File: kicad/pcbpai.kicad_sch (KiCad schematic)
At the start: 16 parts, among them J1 Fuse, J2 Conn_01x04_Pin, J3 Input 24 V, J4 Boton Encendido, J5 Parada de Emergencia, J6 Conn_01x06_Pin, J7 Raspberry GPIO, J8 Conn_01x09_Pin, J9 Conn_01x02_Socket, SW1 SW_Push_DPDT, U6 ATtiny85-20P

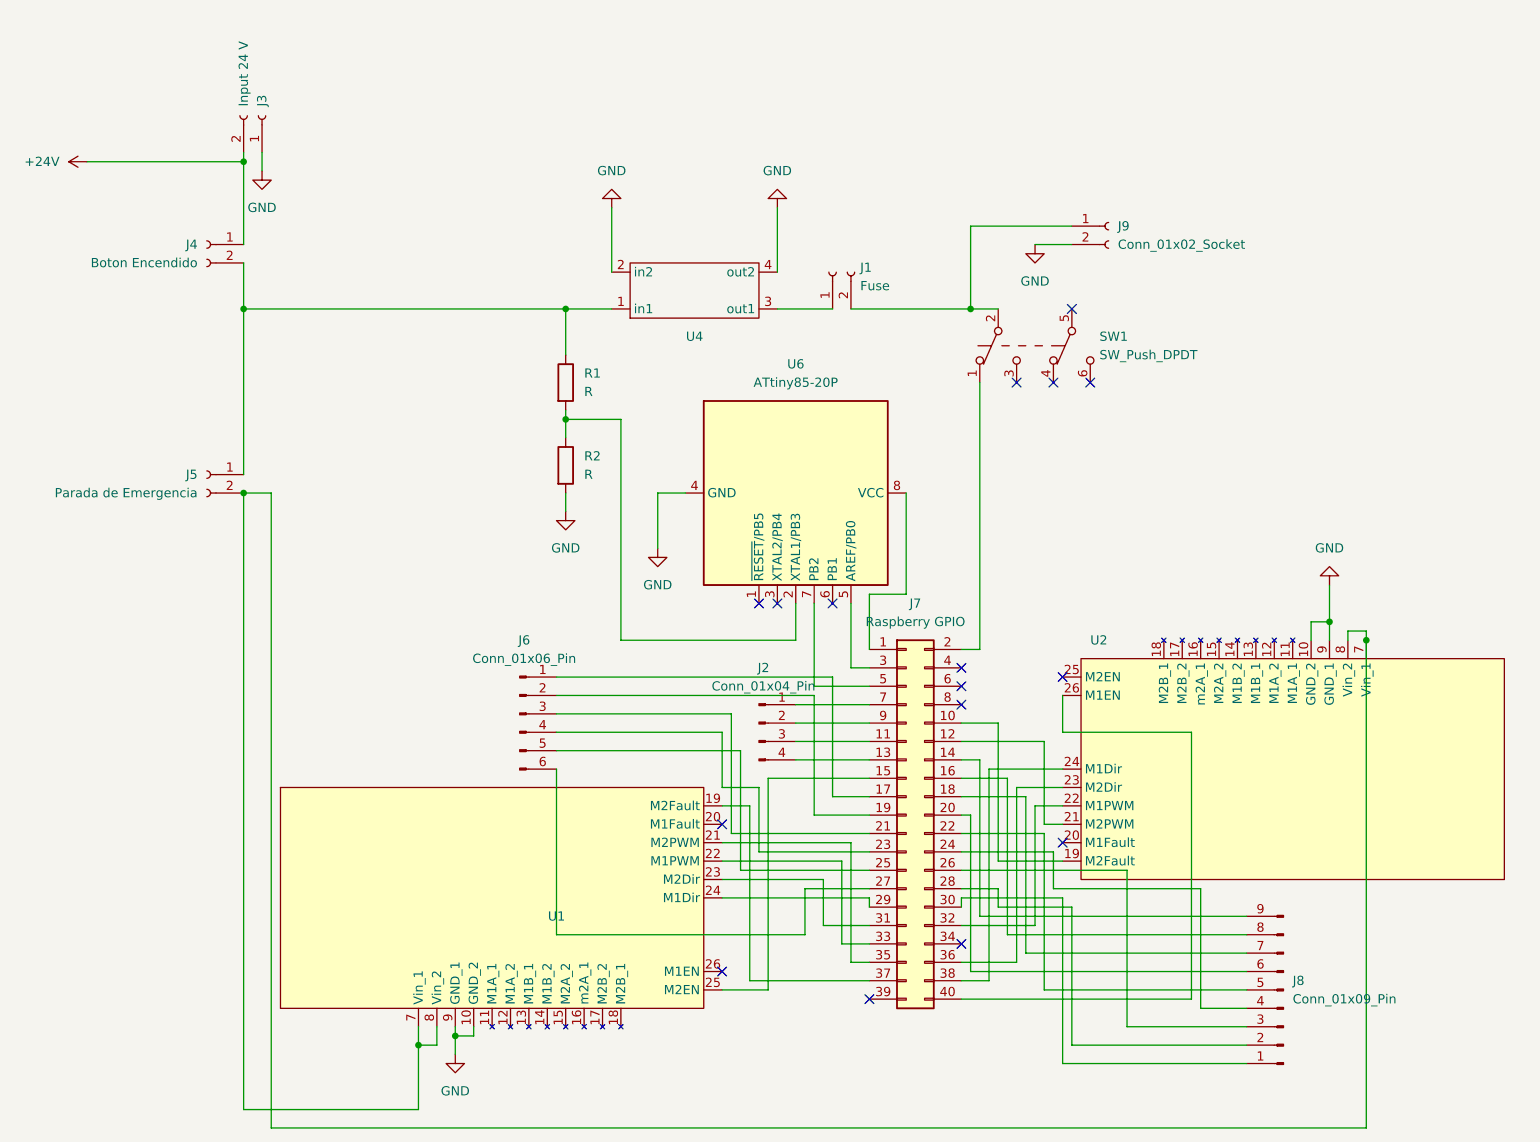
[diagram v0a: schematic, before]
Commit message: finish pcb
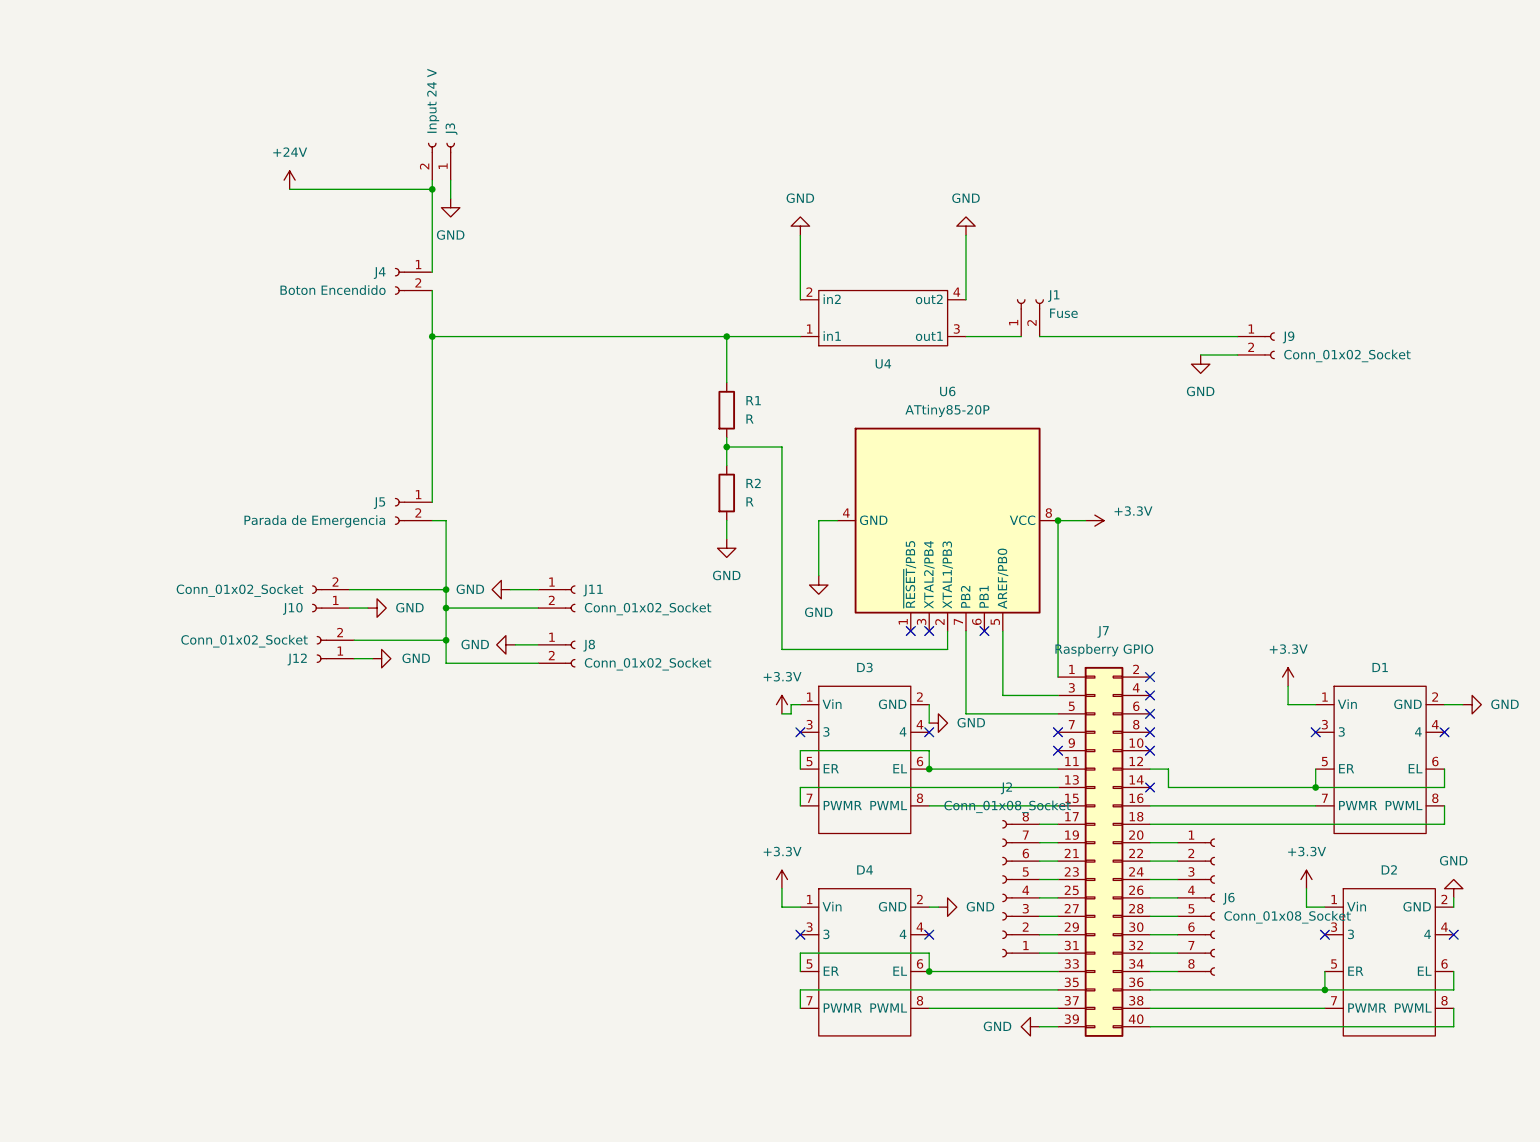
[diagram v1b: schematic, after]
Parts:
- removed J2: Conn_01x04_Pin, Connector_PinSocket_2.54mm:PinSocket_1x04_P2.54mm_Vertical, symbol Connector:Conn_01x04_Pin
- removed J6: Conn_01x06_Pin, Connector_PinSocket_2.54mm:PinSocket_1x06_P2.54mm_Vertical, symbol Connector:Conn_01x06_Pin
- removed J8: Conn_01x09_Pin, Connector_PinSocket_2.54mm:PinSocket_1x09_P2.54mm_Vertical, symbol Connector:Conn_01x09_Pin
- removed SW1: SW_Push_DPDT, PAI:switch, symbol Switch:SW_Push_DPDT
- removed U1, U2: ~, PAI:Pololu MAX 14870 Dual Shield Arduino, symbol Lib_PAI:Dual_MAX14870
- added D1, D2, D3, D4: ~, Connector_PinHeader_2.54mm:PinHeader_2x04_P2.54mm_Vertical, symbol Lib_PAI:Conector_2x4
- added J10, J11, J12, J8: Conn_01x02_Socket, Connector_Phoenix_MSTB:PhoenixContact_MSTBA_2,5_2-G_1x02_P5.00mm_Horizontal, symbol Connector:Conn_01x02_Socket
- added J2, J6: Conn_01x08_Socket, Connector_PinSocket_2.54mm:PinSocket_1x08_P2.54mm_Vertical, symbol Connector:Conn_01x08_Socket
- U4: footprint PAI:regulador -> PAI:regulator
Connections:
- net GND: now also J7.39 (Pin_39), D1.2 (GND), D2.2 (GND), D3.2 (GND), D4.2 (GND), J10.1 (Pin_1), J11.1 (Pin_1), J12.1 (Pin_1), J8.1 (Pin_1)
- net at J5.2 (Pin_2): now also J10.2 (Pin_2), J11.2 (Pin_2), J12.2 (Pin_2), J8.2 (Pin_2)
- net at J7.37 (Pin_37): now also D4.8 (PWML)
- net at J7.35 (Pin_35): now also D4.7 (PWMR)
- net at J7.33 (Pin_33): now also D4.5 (ER), D4.6 (EL)
- net at J7.31 (Pin_31): now also J2.1 (Pin_1)
- net at J7.29 (Pin_29): now also J2.2 (Pin_2)
- net at J7.15 (Pin_15): now also D3.8 (PWML)
- net at J7.12 (Pin_12): now also D1.5 (ER), D1.6 (EL)
- net at J7.32 (Pin_32): now also J6.7 (Pin_7)
- net at J7.36 (Pin_36): now also D2.5 (ER), D2.6 (EL)
- net at J7.38 (Pin_38): now also D2.7 (PWMR)
- net at J7.40 (Pin_40): now also D2.8 (PWML)
- net +3.3V: now reaches J7.1 (Pin_1), U6.8 (VCC)
- net +3.3V: now also D1.1 (Vin), D2.1 (Vin), D3.1 (Vin), D4.1 (Vin)
- net at J7.11 (Pin_11): now also D3.5 (ER), D3.6 (EL)
- net at J7.13 (Pin_13): now also D3.7 (PWMR)
- net at J7.16 (Pin_16): now also D1.7 (PWMR)
- net at J7.17 (Pin_17): now also J2.8 (Pin_8)
- net at J7.18 (Pin_18): now also D1.8 (PWML)
- net at J7.19 (Pin_19): now also J2.7 (Pin_7)
- net at J7.20 (Pin_20): now also J6.1 (Pin_1)
- net at J7.21 (Pin_21): now also J2.6 (Pin_6)
- net at J7.22 (Pin_22): now also J6.2 (Pin_2)
- net at J7.23 (Pin_23): now also J2.5 (Pin_5)
- net at J7.24 (Pin_24): now also J6.3 (Pin_3)
- net at J7.25 (Pin_25): now also J2.4 (Pin_4)
- net at J7.26 (Pin_26): now also J6.4 (Pin_4)
- net at J7.27 (Pin_27): now also J2.3 (Pin_3)
- net at J7.28 (Pin_28): now also J6.5 (Pin_5)
- net at J7.30 (Pin_30): now also J6.6 (Pin_6)
- net at J7.34 (Pin_34): now also J6.8 (Pin_8)
- no-connect marks 16 -> 19
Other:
- moved on the sheet: J1, J3, J4, J5, J7, J9, R1, R2, U4, U6

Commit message: add gerber files and change footprints
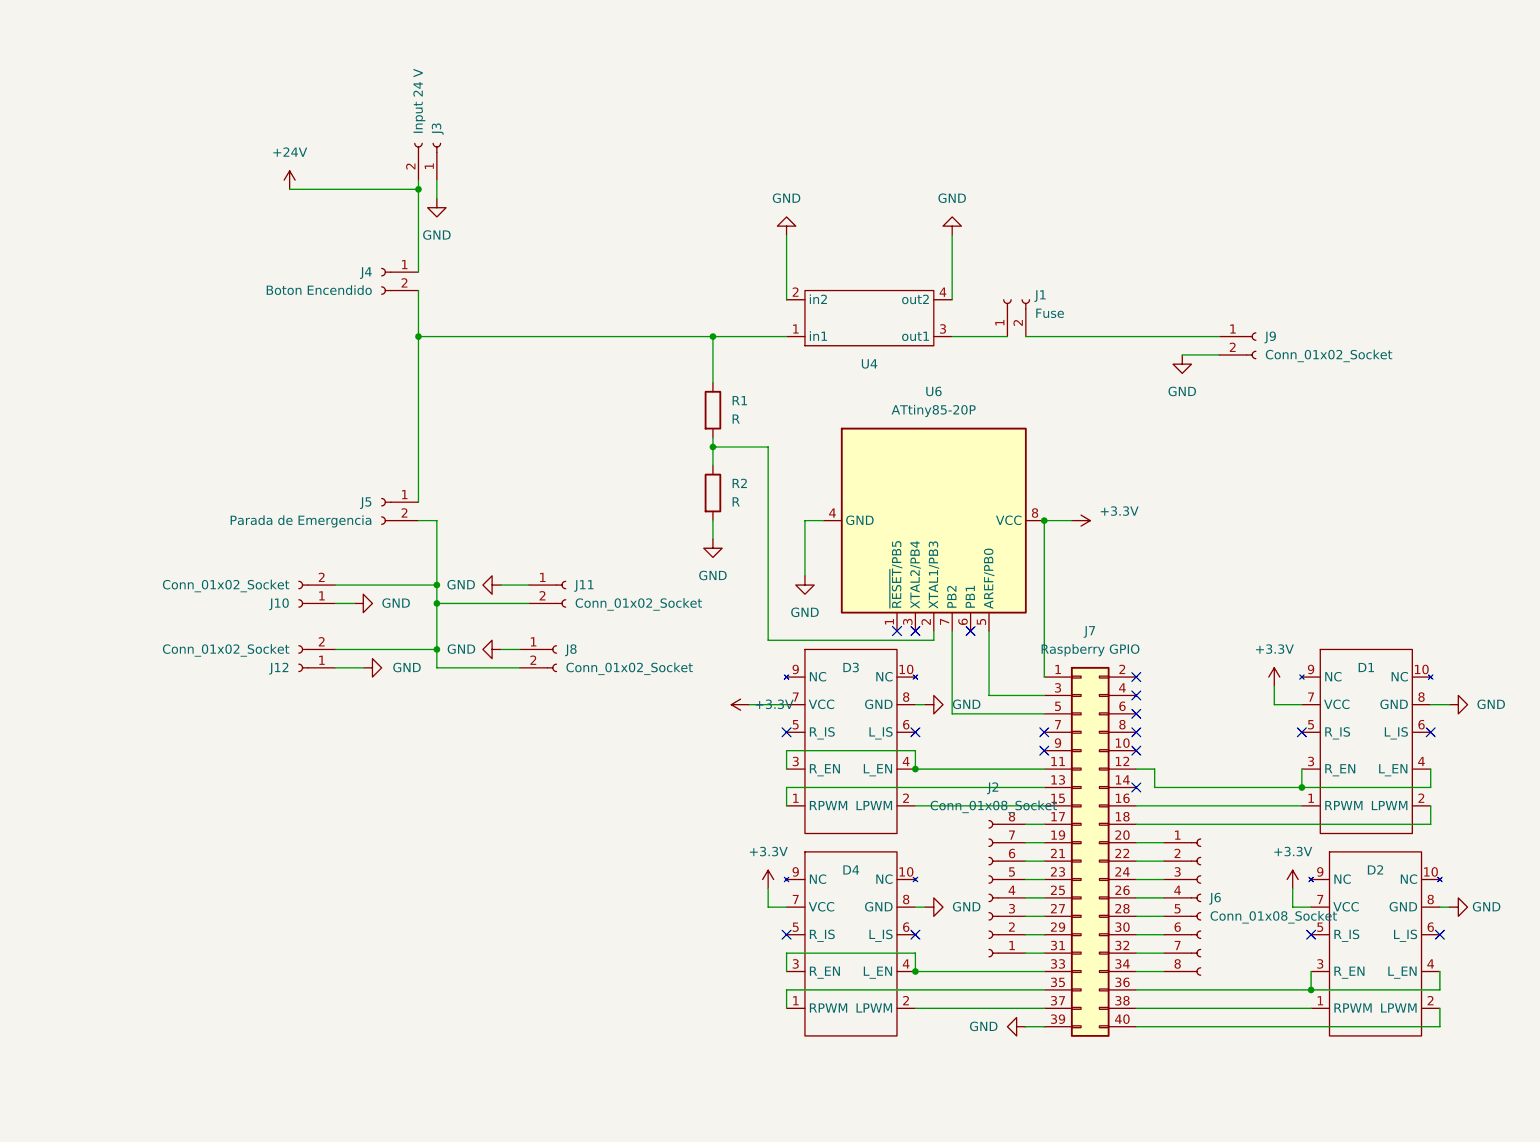
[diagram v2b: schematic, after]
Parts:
- D1, D2, D3, D4: footprint Connector_PinHeader_2.54mm:PinHeader_2x04_P2.54mm_Vertical -> Connector_IDC:IDC-Header_2x05_P2.54mm_Vertical; symbol Lib_PAI:Conector_2x4 -> Lib_PAI:BTS7960_control_pins
- J7: footprint Connector_PinHeader_2.54mm:PinHeader_2x20_P2.54mm_Vertical -> Connector_IDC:IDC-Header_2x20_P2.54mm_Vertical
- U4: symbol Lib_PAI:Regulador -> Lib_PAI:Regulator
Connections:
- net +3.3V: now also D1.7 (VCC), D2.7 (VCC), D3.7 (VCC), D4.7 (VCC); no longer D1.1 (Vin), D2.1 (Vin), D3.1 (Vin), D4.1 (Vin)
- net GND: now also D1.8 (GND), D2.8 (GND), D3.8 (GND), D4.8 (GND); no longer D1.2 (GND), D2.2 (GND), D3.2 (GND), D4.2 (GND)
- net at D1.3 (R_EN): now also D1.4 (L_EN), J7.12 (Pin_12)
- net at J7.16 (Pin_16): now also D1.1 (RPWM); no longer D1.7 (PWMR)
- net at J7.18 (Pin_18): now also D1.2 (LPWM); no longer D1.8 (PWML)
- net at D2.3 (R_EN): now also D2.4 (L_EN), J7.36 (Pin_36)
- net at J7.38 (Pin_38): now also D2.1 (RPWM); no longer D2.7 (PWMR)
- net at J7.40 (Pin_40): now also D2.2 (LPWM); no longer D2.8 (PWML)
- net at J7.13 (Pin_13): now also D3.1 (RPWM); no longer D3.7 (PWMR)
- net at J7.15 (Pin_15): now also D3.2 (LPWM); no longer D3.8 (PWML)
- net at J7.35 (Pin_35): now also D4.1 (RPWM); no longer D4.7 (PWMR)
- net at J7.37 (Pin_37): now also D4.2 (LPWM); no longer D4.8 (PWML)
- net at D4.3 (R_EN): now also D4.4 (L_EN), J7.33 (Pin_33)
- net at D3.3 (R_EN): now also D3.4 (L_EN), J7.11 (Pin_11)
- now unconnected: D1.5 (ER), D1.6 (EL), D2.5 (ER), D2.6 (EL), D3.5 (ER), D3.6 (EL), D4.5 (ER), D4.6 (EL)
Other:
- moved on the sheet: J1, J10, J11, J12, J2, J3, J4, J5, J6, J7, J8, J9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
